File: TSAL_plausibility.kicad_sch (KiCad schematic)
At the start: 32 parts, among them Q1 NMOS, U10 SN74HCS266PWR, U12 74LVC1G32GV, U14 OPA355NA, U3 74LVC2G74, U6 CD74HC30PWR, U7 4072, U8 4001, U9 74LVC1G32GV

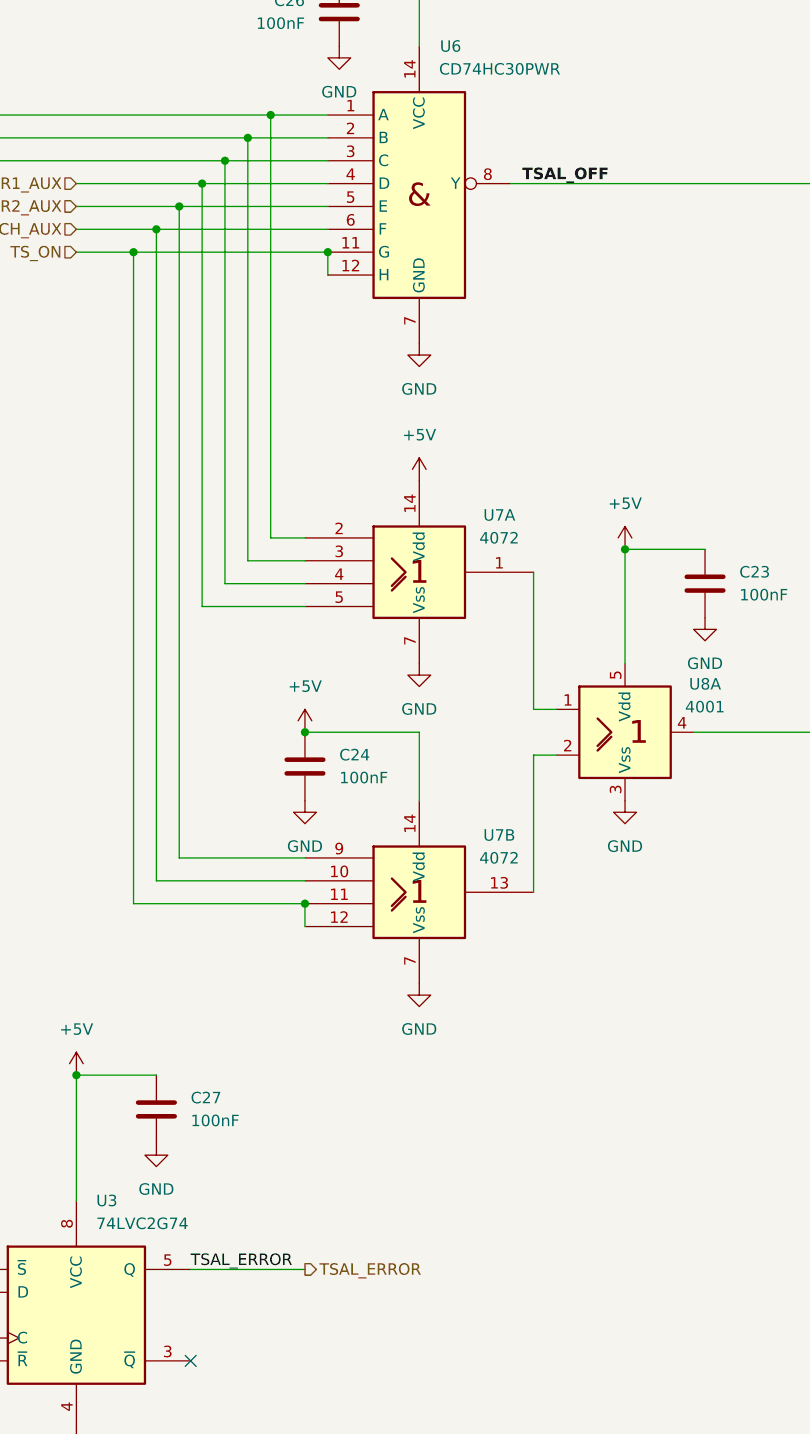
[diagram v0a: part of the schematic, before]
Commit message: Submission Ready. ESF 15.07.24
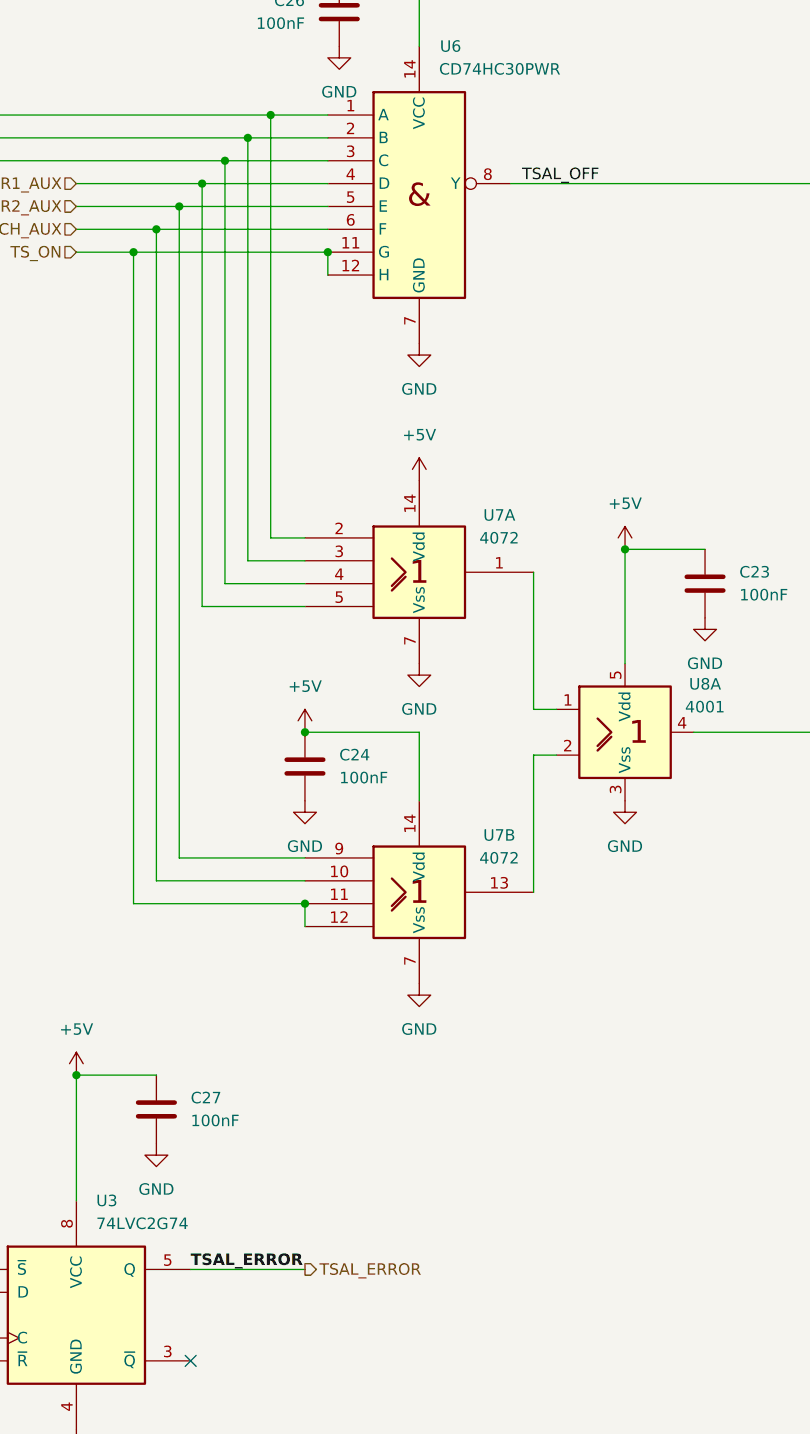
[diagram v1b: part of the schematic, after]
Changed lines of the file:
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@@
 			(font
 				(size 1.27 1.27)
+				(bold yes)
 			)
 			(justify left bottom)
@@
 			(font
 				(size 1.27 1.27)
-				(bold yes)
 			)
 			(justify left bottom)

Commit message: ⠀⠀⠀⠀⠀⠀⠀⠀⠀⠀⠀⠀⠀⠀⠀⠀⠀⠀⠀⠀⠀⠀⠀⠀⠀⠀⠀⠀⠀⠀⠀⠀⠀⠀⠀⠀⠀⣠⣤⣤⣤⡀⠀⠀⠀⠀⠀⠀⠀⠀⠀⠀⠀⠀⠀⠀⠀⠀⠀⠀⠀⠀⠀⠀⠀ ⠀⠀⠀⠀⠀⠀⠀⠀⠀⠀⠀⠀⠀⠀⠀⠀⠀⠀⠀⠀⠀⠀⠀⠀⠀⠀⠀⠀⠀⠀⠀⠀⠀⠀⣠⣶⣿⠟⠉⠉⠻⣿⡄⠀⠀⠀⠀⠀⠀⠀⠀⠀⠀⠀⠀⠀⠀⠀⠀⠀⠀⠀⠀⠀⠀ ⠀⠀⠀⠀⠀⠀⠀⠀⠀⠀⠀⠀⠀⠀⠀⠀⠀⠀⠀⠀⠀⠀⠀⠀⠀⠀⠀⠀⠀⠀⠀⢀⣤⣾⠿⠉⠀⠀⠀⠀⠀⠹⣿⡄⠀⠀⠀⠀⠀⠀⠀⠀⠀⠀⠀⠀⠀⠀⠀⠀⠀⠀⣀⣴⣾ ⠀⠀⠀⠀⠀⠀⠀⠀⠀⠀⠀⠀⠀⠀⠀⠀⠀⠀⠀⠀⠀⠀⠀⠀⠀⠀⠀⠀⠀⢀⣴⣿⠟⠁⠀⠀⠀⠀⠀⠀⠀⠀⣿⣿⠀⠀⠀⠀⠀⠀⠀⠀⠀⠀⠀⠀⠀⠀⠀⣀⣴⣾⡿⠛⠉ ⠀⠀⠀⠀⠀⠀⠀⠀⠀⠀⠀⠀⠀⠀⠀⠀⠀⠀⠀⠀⠀⠀⠀⠀⠀⠀⠀⢀⣴⣿⠟⠁⠀⠀⠀⠀⠀⠀⠀⠀⠀⠀⢸⣿⡆⠀⠀⠀⠀⠀⠀⠀⠀⠀⠀⠀⢀⣴⣾⡿⠟⠁⠀⠀⠀ ⠀⠀⠀⠀⠀⠀⠀⠀⠀⠀⠀⠀⠀⠀⠀⠀⠀⠀⠀⠀⠀⠀⠀⠀⢀⣀⣴⣿⡿⠃⠀⠀⠀⠀⠀⠀⠀⠀⠀⠀⠀⠀⢸⣿⣷⣶⣶⣦⣤⣤⣄⡀⠀⢀⣠⣾⣿⠿⠋⠀⠀⠀⠀⠀⣠ ⠀⠀⠀⠀⠀⠀⠀⠀⠀⠀⠀⠀⠀⠀⠀⠀⠀⠀⠀⠀⠀⠀⠀⣼⣿⣿⡿⠋⠀⠀⠀⠀⠀⠀⠀⠀⠀⠀⠀⣠⣤⠶⠞⣿⠟⠋⠉⠉⠙⣻⠿⢿⣿⣿⣿⠟⠁⠀⠀⠀⠀⠀⢀⡼⠁ ⠀⠀⠀⠀⠀⠀⠀⠀⠀⠀⠀⠀⠀⠀⠀⠀⠀⠀⠀⠀⠀⠀⢰⣿⠁⠛⠀⠀⠀⠀⠀⠀⠀⠀⠀⠀⠀⠀⣰⠟⠁⢠⡞⠁⠀⠀⠀⢀⡴⠋⠀⢀⡿⠋⠁⠀⠀⠀⠀⠀⠀⠀⡞⠁⠀ ⠀⠀⠀⠀⠀⠀⠀⠀⠀⠀⠀⠀⠀⠀⠀⠀⠀⠀⠀⠀⠀⣠⣼⣿⡄⠀⠀⠀⠀⠀⠀⠀⠀⠀⠀⠀⠀⣼⠃⠀⢠⠏⠀⠀⠀⠀⣰⠏⠀⠀⣠⠟⠀⠀⠀⠀⠀⠀⠀⠀⠀⢸⡥⠤⡀ ⠀⠀⠀⠀⠀⠀⠀⠀⠀⠀⠀⠀⠀⠀⠀⠀⠀⠀⠀⠀⣰⣿⠟⠁⠀⠀⠀⠀⠀⠀⠀⠀⠀⠀⠀⠀⠠⣇⠀⣠⡏⠀⠀⠀⠀⣼⠁⠀⠀⣰⠋⠀⠀⠀⠀⠀⠀⠀⠀⠀⠀⠀⢀⡴⠁ ⠀⠀⠀⠀⠀⠀⠀⠀⠀⠀⠀⠀⠀⠀⠀⠀⣀⣄⣄⣼⣿⠋⠀⠀⠀⠀⠀⠀⠀⠀⠀⠀⠀⠀⠀⠀⠀⢻⡶⠋⠀⠀⠀⠀⢸⣧⠀⠀⣴⠃⠀⠀⠀⠀⠀⠀⠀⠀⠀⠀⠀⠀⠘⢧⠀ ⠀⠀⠀⠀⠀⠀⠀⠀⢀⣀⣀⠀⠀⠀⠀⣾⡿⠿⣿⡿⠁⠀⠀⠀⠀⠀⠀⣠⣶⣶⣶⡀⠀⠀⠀⠀⠀⠀⠀⠀⠀⠀⠀⠀⠀⠙⠛⠛⠁⠀⠀⠀⠀⠀⠀⠀⠀⠀⠀⠀⠀⠀⠀⠈⠳ ⠀⠀⠀⠀⠀⠀⢀⣾⠿⠛⢿⣿⣷⣄⡀⣿⠃⠀⠈⠀⠀⠀⠀⠀⠀⢀⣾⣿⣿⣿⣿⣧⠀⠀⠀⠀⠀⠀⠀⠀⠀⠀⠀⠀⠀⠀⠀⠀⠀⠀⠀⠀⠀⠀⠀⠀⠀⠀⠀⠀⠀⠀⠀⠀⠀ ⠀⠀⠀⣠⣤⣦⣼⣿⠀⠀⠀⣿⣿⣿⣿⣿⣦⣀⠀⠀⠀⠀⠀⠀⠀⣿⣿⣿⣿⣿⣿⡿⠀⠀⠀⢀⣀⣀⣀⣀⡀⠀⠀⠀⠀⠀⠀⠀⠀⠀⠀⣤⣾⣿⣿⣿⣷⣄⠀⠀⠀⠀⠀⠀⠀ ⠀⣠⣾⡿⠋⠉⠉⠁⠀⠀⠀⠀⠉⢯⡙⠻⣿⣿⣷⣤⡀⠀⠀⠀⠀⢿⣿⣿⣿⣿⡿⠃⢀⡤⠖⠋⠉⠉⠉⠉⠉⠉⠒⠦⣄⠀⠀⠀⠀⠀⣾⣿⣿⣿⣿⣿⣿⣿⣧⠀⠀⠀⠀⠀⠀ ⣾⣿⠋⠀⠀⠀⠀⣀⣀⠀⠀⠀⠀⠀⠙⢦⣄⠉⠻⢿⣿⣷⣦⡀⠀⠈⠙⠛⠛⠋⠀⢰⠟⡇⠀⠀⠀⠀⠀⠀⠀⠀⠀⠀⠈⠳⣄⠀⠀⠀⣿⣿⣿⣿⣿⣿⣿⣿⣿⠀⠀⠀⠀⠀⠀ ⣿⡇⠀⠀⠀⣴⠟⣫⣿⣿⣄⠀⠀⠀⠀⡶⢌⡙⠶⣤⡈⠛⠿⣿⣷⣦⣀⠀⠀⠀⠀⡇⠀⢻⣄⠀⠀⣠⢷⠀⠀⠀⠀⠀⡶⠀⠘⡆⠀⠀⠻⣿⣿⣿⣿⣿⣿⣿⡟⠀⠀⠀⠀⠀⠀ ⣿⡇⠀⠀⢸⣟⢸⣿⣿⣿⣿⠀⠀⠀⠀⡇⠀⠈⠛⠦⣝⡳⢤⣈⠛⠻⣿⣷⣦⣀⠀⠀⠀⠀⠈⠙⠋⠁⠀⠛⠦⠤⠤⠚⠁⠀⠀⢳⠀⠀⠀⠈⠛⠿⠿⠿⠟⠋⠀⠀⠀⠀⠀⠀⠀ ⣿⡇⠀⠀⠈⢿⣞⣿⣿⣿⠏⠀⠀⠀⠀⡇⠀⠀⠀⠀⠀⠙⠳⢬⣛⠦⠀⠙⢻⣿⣷⣦⣀⠀⠀⠀⠀⠀⠀⠀⠀⠀⠀⠀⠀⠀⠀⡞⠀⠀⠀⠀⠀⠀⠀⠀⠀⠀⠀⠀⠀⠀⠀⠀⠀ ⣿⡇⠀⠀⠀⠀⠉⠛⠋⠁⠀⠀⠀⠀⠀⡇⠀⠀⠀⠀⠀⠀⠀⠀⠈⠁⠀⠀⠈⣿⠉⢻⣿⣷⣦⣀⠀⠀⠀⠀⠀⠀⠀⠀⠀⢀⡼⠁⠀⠀⠀⠀⠀⠀⠀⠀⠀⠀⠀⠀⠀⠀⠀⠀⠀ ⣿⡇⠀⠀⠀⠀⠀⣠⣄⠀⠀⢰⠶⠒⠒⢧⣄⡀⠀⠀⠀⠀⠀⠀⠀⠀⠀⠀⠀⣿⠀⢸⡇⢸⡟⢿⣷⣦⣴⣶⣶⣶⣶⣤⣔⠋⠀⠀⠀⠀⠀⠀⠀⠀⠀⠀⠀⠀⠀⠀⠀⠀⠀⠀⠀ ⣿⡇⠀⠀⣤⠀⠀⠿⠿⠁⢀⡿⠀⠀⠀⡄⠈⠙⡷⢦⣄⡀⠀⠀⠀⠀⠀⠀⠀⣿⠀⢸⡇⢸⡇⠀⣿⠙⣿⣿⣉⠉⠙⠿⣿⣧⠀⠀⠀⠀⠀⠀⠀⠀⠀⠀⠀⠀⠀⠀⠀⠀⠀⠀⠀ ⣿⡇⠀⠀⠙⠷⢤⣀⣠⠴⠛⠁⠀⠀⠀⠇⠀⠀⡇⢸⡏⢹⡷⢦⣄⡀⠀⠀⠀⣿⡀⢸⡇⢸⡇⠀⡟⠀⢸⠀⢹⡷⢦⣄⣘⣿⡆⠀⠀⠀⠀⠀⠀⠀⠀⠀⠀⠀⠀⠀⠀⠀⠀⠀⠀ ⣿⣿⠢⣤⡀⠀⠀⠀⠀⠀⠀⣠⠾⣿⣿⡷⣤⣀⡇⠸⡇⢸⡇⢸⠉⠙⠳⢦⣄⡻⢿⣾⣧⣸⣧⠀⡇⠀⢸⠀⢸⡇⢤⣈⠙⠻⣿⣆⠀⠀⠀⠀⠀⠀⠀⠀⠀⠀⠀⠀⠀⠀⠀⠀⠀ ⢹⣿⣷⣌⡉⠛⠲⢶⣶⠖⠛⠛⢶⣄⡉⠛⠿⣽⣿⣶⣧⣸⡇⢸⠀⠀⠀⠀⠈⠙⠲⢮⣝⠻⣿⣷⣷⣄⣸⠀⢸⡇⠀⠈⠁⠀⢸⣿⠀⠀⠀⠀⠀⠀⠀⠀⠀⠀⠀⠀⠀⠀⠀⠀⠀ ⠀⠈⠙⠻⢿⣷⣶⣤⣉⡻⢶⣄⣀⠈⠙⠳⢦⣈⡉⠻⢿⣿⣷⣾⣦⡀⠀⠀⠀⠀⠀⠀⠈⠙⠲⢭⣛⠿⣿⣷⣼⡇⠀⠀⠀⠀⠈⣿⡇⠀⠀⠀⠀⠀⠀⣀⠀⠀⠀⠀⠀⠀⠀⠀⣀ ⠀⠀⠀⠀⠀⠈⠙⠻⢿⣿⣷⣶⣽⣻⡦⠀⠀⠈⠙⠷⣦⣌⡙⠻⢿⣟⣷⣤⣀⠀⠀⠀⠀⠀⠀⠀⠈⠙⠳⢯⣻⡇⠀⠀⠀⠀⠀⢸⣿⠀⣀⠀⠀⠀⠀⠈⠳⣄⠀⠀⠀⢀⡏⠙⠛ ⠀⠀⠀⠀⠀⠀⠀⠀⠀⠈⠛⠻⢿⣿⣿⣿⣶⣤⣤⣤⣀⣈⠛⠷⣤⣈⡛⠷⢽⡻⢶⣄⣀⠀⠀⠀⠀⠀⠀⠀⠈⠛⠳⢤⣀⠀⠀⢸⣿⡀⠈⠳⢤⣀⣀⣰⠃⠈⠛⠶⠶⠿⠃⠀⠀ ⠀⠀⠀⠀⠀⠀⠀⠀⠀⠀⠀⠀⠀⢈⣿⡿⠛⠉⠙⠛⠛⠻⢷⣦⣄⣩⣿⠶⠖⠛⠛⠛⠛⠛⠛⠿⢷⣶⣦⣄⠀⠀⠀⠀⠉⢻⣶⣿⣿⠇⠀⠀⠀⠉⠉⠀⠀⠀⠀⠀⠀⠀⠀⠀⠀ ⠀⠀⠀⠀⠀⠀⠀⠀⠀⠀⠀⠀⠀⣼⣿⠁⠀⠀⠀⠀⠀⠀⠀⣿⣿⠋⠀⠀⠀⠀⠀⣠⠖⠂⠀⠀⠀⠈⠙⠿⣿⣦⡄⠀⠀⣸⣿⠟⠋⠀⠀⠀⠀⠀⠀⠀⠀⠀⠀⠀⠀⠀⠀⠀⠀ ⠀⠀⠀⠀⠀⠀⠀⠀⠀⠀⠀⠀⢰⣿⡟⠀⠀⠀⠀⠀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
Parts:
- C21, C22, C23, C24, C25, C26, C27, C28: footprint (none) -> Capacitor_SMD:C_0603_1608Metric
- Q1: footprint (none) -> Package_TO_SOT_SMD:SOT-23-3
- R28, R84, R87, R88, R89, R90: footprint (none) -> Resistor_SMD:R_0603_1608Metric
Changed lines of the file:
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@@
 			)
 		)
-		(property "Footprint" ""
+		(property "Footprint" "Capacitor_SMD:C_0603_1608Metric"
 			(at 229.5652 87.63 0)
 			(effects
@@
 			)
 		)
-		(property "Footprint" ""
+		(property "Footprint" "Capacitor_SMD:C_0603_1608Metric"
 			(at 218.7448 34.29 0)
 			(effects
@@
 			)
 		)
-		(property "Footprint" ""
+		(property "Footprint" "Capacitor_SMD:C_0603_1608Metric"
 			(at 72.0852 144.78 0)
 			(effects
@@
 			)
 		)
-		(property "Footprint" ""
+		(property "Footprint" "Resistor_SMD:R_0603_1608Metric"
 			(at 52.578 40.64 90)
 			(effects
@@
 			)
 		)
-		(property "Footprint" ""
+		(property "Footprint" "Capacitor_SMD:C_0603_1608Metric"
 			(at 129.2352 148.59 0)
 			(effects
@@
 			)
 		)
-		(property "Footprint" ""
+		(property "Footprint" "Package_TO_SOT_SMD:SOT-23-3"
 			(at 270.51 41.91 0)
 			(effects
@@
 			)
 		)
-		(property "Footprint" ""
+		(property "Footprint" "Resistor_SMD:R_0603_1608Metric"
 			(at 44.45 99.568 90)
 			(effects
@@
 			)
 		)
-		(property "Footprint" ""
+		(property "Footprint" "Resistor_SMD:R_0603_1608Metric"
 			(at 52.578 69.85 90)
 			(effects
@@
 			)
 		)
-		(property "Footprint" ""
+		(property "Footprint" "Capacitor_SMD:C_0603_1608Metric"
 			(at 147.6248 26.67 0)
 			(effects
@@
 			)
 		)
-		(property "Footprint" ""
+		(property "Footprint" "Resistor_SMD:R_0603_1608Metric"
 			(at 52.578 101.6 90)
 			(effects
@@
 			)
 		)
-		(property "Footprint" ""
+		(property "Footprint" "Resistor_SMD:R_0603_1608Metric"
 			(at 44.45 38.608 90)
 			(effects
@@
 			)
 		)
-		(property "Footprint" ""
+		(property "Footprint" "Resistor_SMD:R_0603_1608Metric"
 			(at 44.45 67.818 90)
 			(effects
@@
 			)
 		)
-		(property "Footprint" ""
+		(property "Footprint" "Capacitor_SMD:C_0603_1608Metric"
 			(at 265.1252 88.9 0)
 			(effects
@@
 			)
 		)
-		(property "Footprint" ""
+		(property "Footprint" "Capacitor_SMD:C_0603_1608Metric"
 			(at 145.7452 110.49 0)
 			(effects
@@
 			)
 		)
-		(property "Footprint" ""
+		(property "Footprint" "Capacitor_SMD:C_0603_1608Metric"
 			(at 190.1952 90.17 0)
 			(effects
